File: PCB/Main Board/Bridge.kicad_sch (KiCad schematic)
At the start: 46 parts, among them K401 AGQ200A12, Q401 2N4401, Q402 2N4403, Q403 2N4401, Q404 2N4403, U401 OPA2197xD, U402 DG201, U403 OPA2197xD, U404 OPA2197xD

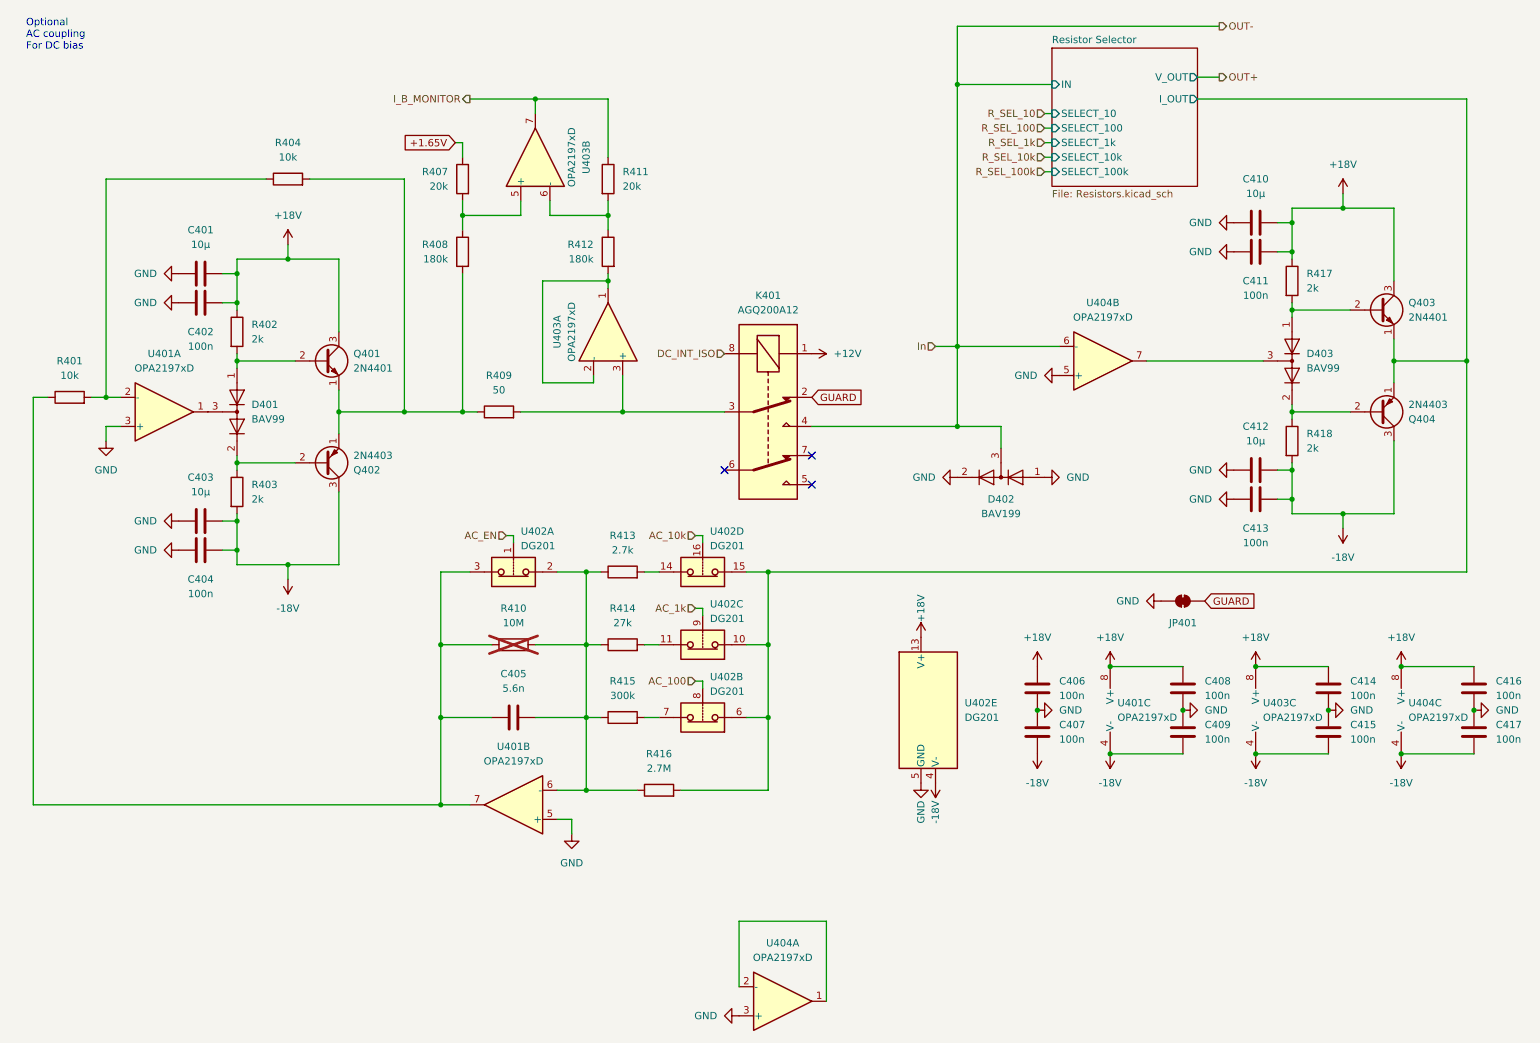
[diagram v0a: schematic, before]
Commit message: minor schematic changes
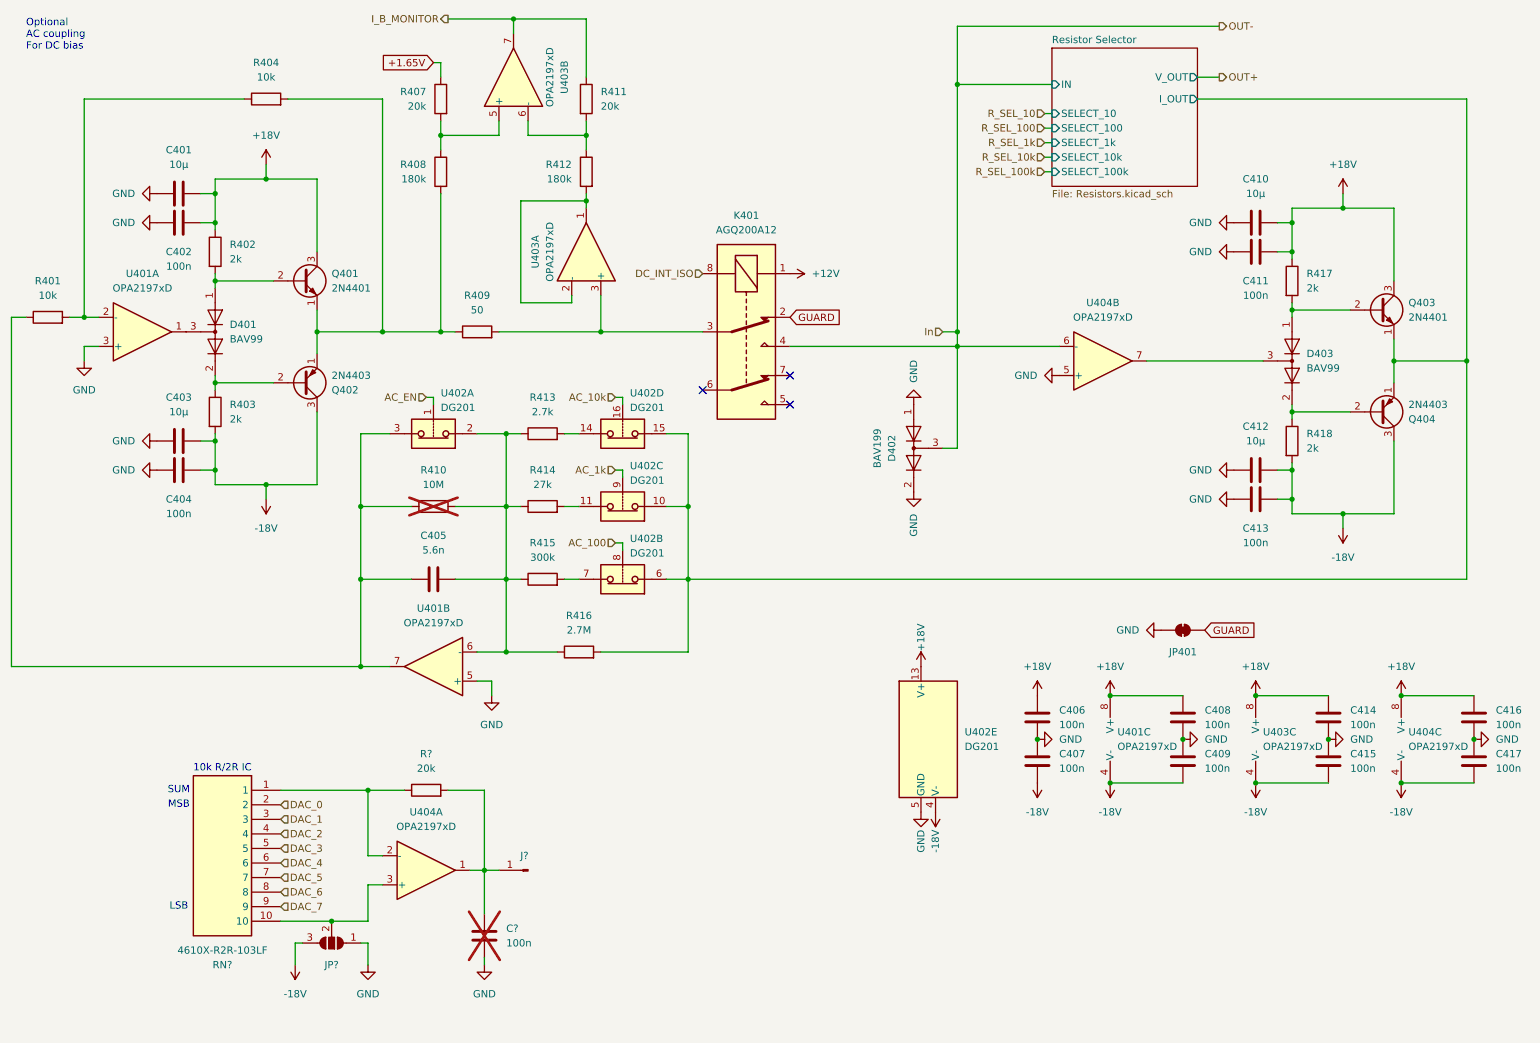
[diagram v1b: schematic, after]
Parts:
- added C?: 100n, Capacitor_SMD:C_0805_2012Metric, symbol Device:C
- added J?: Conn_01x01_Pin, Connector_PinHeader_2.54mm:PinHeader_1x01_P2.54mm_Horizontal, symbol Connector:Conn_01x01_Pin
- added JP?: SolderJumper_3_Open, symbol Jumper:SolderJumper_3_Open
- added R?: 20k, Resistor_SMD:R_0805_2012Metric, symbol Device:R
- added RN?: 4610X-R2R-103LF, SIP249W51P254L2535H508Q10P, symbol 4610X-R2R-103LF:4610X-R2R-103LF
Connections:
- net -18V: now also JP?.3 (B)
- net GND: now also C?.2, JP?.1 (A); no longer U404.3 (+)
- net at U404.2 (-): now also R?.1, RN?.1; no longer U404.1
- new net: JP?.2 (C), RN?.10, U404.3 (+)
- new net: C?.1, J?.1 (Pin_1), R?.2, U404.1
- new net DAC_0: RN?.2
- new net DAC_1: RN?.3
- new net DAC_2: RN?.4
- new net DAC_3: RN?.5
- new net DAC_4: RN?.6
- new net DAC_5: RN?.7
- new net DAC_6: RN?.8
- new net DAC_7: RN?.9
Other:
- note added: "10k R/2R IC"
- note added: "LSB"
- note added: "MSB"
- note added: "SUM"
- moved on the sheet: C401, C402, C403, C404, C405, C406, C407, C408, C409, C414, C415, C416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
